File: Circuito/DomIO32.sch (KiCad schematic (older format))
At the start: 51 parts, among them J2 ICSP, J3 OSTTC032162, J4 OSTTC032162, J5 Conector2X5, SW1 TactSwitch, U1 LM1117-3.3, U2 PIC32MM0064GPL028-I-SO, U3 ESP-02, X1 X, X2 X, X3 X

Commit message: Correccion
Se agrega la conexion del pin 6 del modulo wifi
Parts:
- U2: symbol DomIO32:PIC32MM0064GPL028-I-SO -> DomIO32-rescue:PIC32MM0064GPL028-I-SO-DomIO32
- U3: symbol DomIO32:ESP-02 -> DomIO32-rescue:ESP-02-DomIO32
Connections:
- wire segments 195 -> 197
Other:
- moved on the sheet: C13
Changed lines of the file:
@@
 EESchema Schematic File Version 4
-LIBS:DomIO32-cache
-EELAYER 26 0
+EELAYER 30 0
 EELAYER END
 $Descr A4 11693 8268
@@
 $EndDescr
 $Comp
-L DomIO32:ESP-02 U3
+L DomIO32-rescue:ESP-02-DomIO32 U3
 U 1 1 5DCB6F71
 P 7050 1800
@@
 L Device:C C13
 U 1 1 5DCDBD3D
-P 7600 3150
-F 0 "C13" H 7250 3250 50  0000 L CNN
-F 1 "100nf / 50v" H 7000 3150 50  0000 L CNN
-F 2 "Capacitor_SMD:C_0805_2012Metric_Pad1.15x1.40mm_HandSolder" H 7638 3000 50  0001 C CNN
-F 3 "~" H 7600 3150 50  0001 C CNN
-	1    7600 3150
+P 7600 3050
+F 0 "C13" H 7250 3150 50  0000 L CNN
+F 1 "100nf / 50v" H 7000 3050 50  0000 L CNN
+F 2 "Capacitor_SMD:C_0805_2012Metric_Pad1.15x1.40mm_HandSolder" H 7638 2900 50  0001 C CNN
+F 3 "~" H 7600 3050 50  0001 C CNN
+	1    7600 3050
 	1    0    0    -1
 $EndComp
@@
 	7600 3550 7800 3550
 Connection ~ 7600 3550
-Wire Wire Line
-	7600 3550 7600 3300
-Wire Wire Line
-	7600 3000 7600 2850
 Connection ~ 7600 2750
 Connection ~ 5500 3200
@@
 Wire Wire Line
 	7800 2850 7600 2850
-Connection ~ 7600 2850
 Wire Wire Line
 	7600 2850 7600 2750
@@
 	8600 4050 9600 4050
 $Comp
-L DomIO32:PIC32MM0064GPL028-I-SO U2
+L DomIO32-rescue:PIC32MM0064GPL028-I-SO-DomIO32 U2
 U 1 1 5DD039C1
 P 3950 3450
@@
 Wire Wire Line
 	8600 4150 9650 4150
+Wire Wire Line
+	7600 3200 7600 3250
+Wire Wire Line
+	7600 2900 7600 2850
+Connection ~ 7600 2850
+Wire Wire Line
+	7800 3250 7600 3250
+Connection ~ 7600 3250
+Wire Wire Line
+	7600 3250 7600 3550
 $EndSCHEMATC

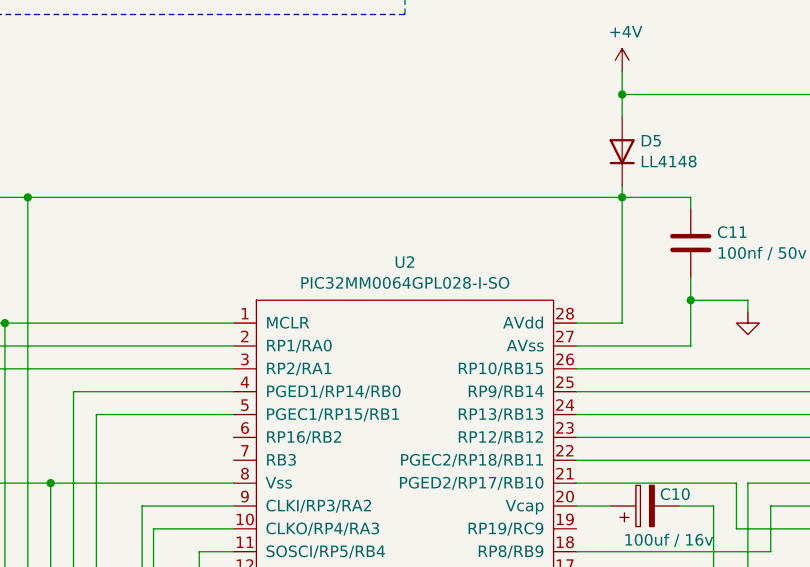
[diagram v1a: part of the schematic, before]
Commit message: Encapsulado PIC
Correcciones al encapsulado del PIC
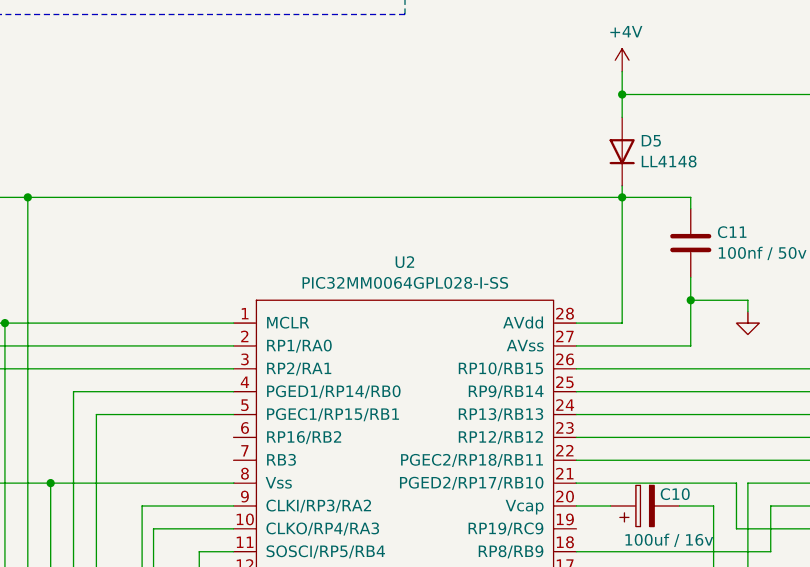
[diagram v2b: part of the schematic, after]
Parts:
- U2: value PIC32MM0064GPL028-I-SO -> PIC32MM0064GPL028-I-SS
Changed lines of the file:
@@
 P 3950 3450
 F 0 "U2" H 4550 3415 50  0000 C CNN
-F 1 "PIC32MM0064GPL028-I-SO" H 4550 3324 50  0000 C CNN
+F 1 "PIC32MM0064GPL028-I-SS" H 4550 3324 50  0000 C CNN
 F 2 "Package_SO:SSOP-28_5.3x10.2mm_P0.65mm" H 3950 3300 50  0001 C CNN
 F 3 "" H 3950 3300 50  0001 C CNN
